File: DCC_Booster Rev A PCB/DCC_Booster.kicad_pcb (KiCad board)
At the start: 2 copper layers, 99.1 x 109.2 mm, 99 parts, among them J1 Conn_01x04, J2 4P4C, J3 4P4C, J4 Prog, J5 Jack-DC, Q1 Q_NMOS_GDS, Q2 Q_NMOS_GDS, Q3 Q_NMOS_GDS, Q4 Q_NMOS_GDS, SW1 SW_DIP_x05, U1 MC34167, U10 LM358, U11 74AHC1G04, U2 R-78E5.0-1.0, U3 74HC08, U4 IR2101, U5 IR2101, U6 74AHC1G04, U7 6N137, U8 PIC16F1847-IP, U9 74AHC1G86

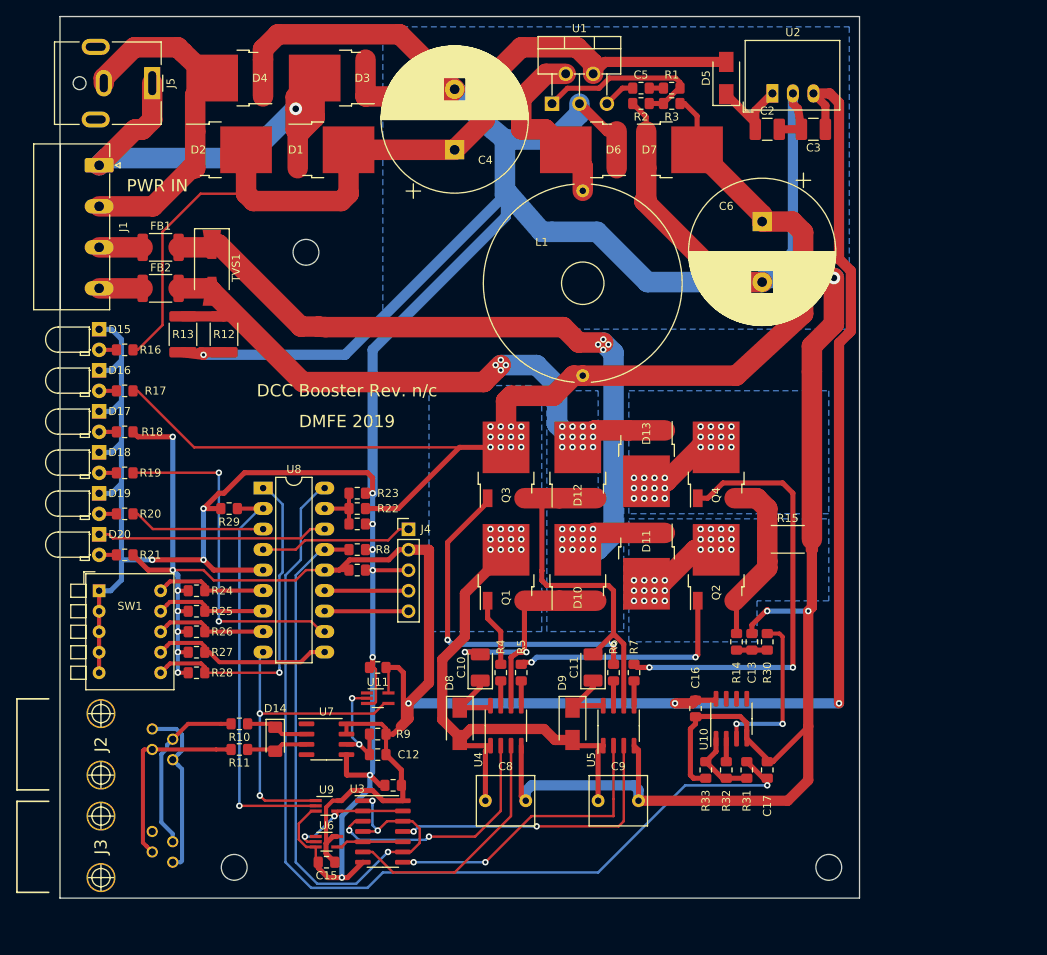
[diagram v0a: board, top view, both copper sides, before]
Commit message: Rev A PCB ordered
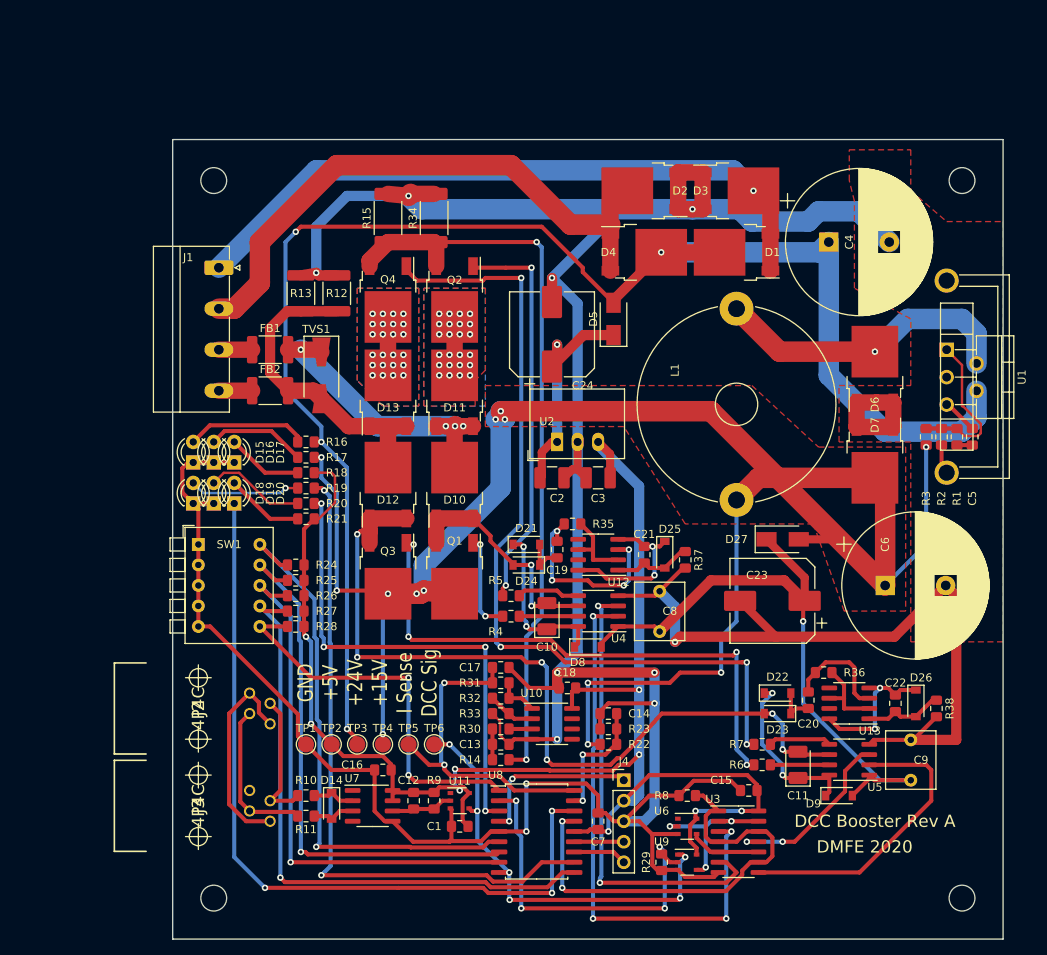
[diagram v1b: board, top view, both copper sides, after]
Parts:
- removed J5: Jack-DC, Connector_BarrelJack:BarrelJack_CUI_PJ-063AH_Horizontal
- added C19: 0.1uf50v, Capacitor_SMD:C_0805_2012Metric_Pad1.15x1.40mm_HandSolder, F.Cu at (97.2, 94.0)
- added C20: 0.1uf50v, Capacitor_SMD:C_0805_2012Metric_Pad1.15x1.40mm_HandSolder, F.Cu at (128.3, 112.6)
- added C21: 0.1uf50v, Capacitor_SMD:C_0805_2012Metric_Pad1.15x1.40mm_HandSolder, F.Cu at (108.0, 94.6)
- added C22: 0.1uf50v, Capacitor_SMD:C_0805_2012Metric_Pad1.15x1.40mm_HandSolder, F.Cu at (139.1, 113.0)
- added C23: 220uF, Capacitor_SMD:CP_Elec_10x10, F.Cu at (123.8, 100.3)
- added C24: 220uF, Capacitor_SMD:CP_Elec_10x10, F.Cu at (96.5, 67.3)
- added D21: 1N4148W, Diode_SMD:D_SOD-123, F.Cu at (93.3, 93.3)
- added D22: 1N4148W, Diode_SMD:D_SOD-123, F.Cu at (124.5, 111.8)
- added D23: 1N4148W, Diode_SMD:D_SOD-123, F.Cu at (124.5, 114.3)
- added D24: 1N4148W, Diode_SMD:D_SOD-123, F.Cu at (93.3, 95.9)
- added D25: BZT52C15, Diode_SMD:D_SOD-123, F.Cu at (110.5, 94.6)
- added D26: BZT52C15, Diode_SMD:D_SOD-123, F.Cu at (141.6, 113.0)
- added D27: MRA4003T3G, Diode_SMD:D_SMA, F.Cu at (125.1, 92.7)
- added H4: MountingHole_3.2mm_M3, MountingHole:MountingHole_3.2mm_M3, F.Cu at (147.3, 137.2)
- added HS1: Heatsink_Fischer_FK224xx2201_25x8.3mm, Heatsink:Heatsink_Fischer_FK224xx2201_25x8.3mm, F.Cu at (145.4, 84.5)
- added R34: 0R10 3W, Resistor_SMD:R_2512_6332Metric_Pad1.52x3.35mm_HandSolder, F.Cu at (81.9, 52.9)
- added R35: 10K, Resistor_SMD:R_0805_2012Metric_Pad1.15x1.40mm_HandSolder, F.Cu at (99.1, 90.8)
- added R36: 10K, Resistor_SMD:R_0805_2012Metric_Pad1.15x1.40mm_HandSolder, F.Cu at (130.2, 109.2)
- added R37: 100, Resistor_SMD:R_0805_2012Metric_Pad1.15x1.40mm_HandSolder, F.Cu at (113.0, 95.2)
- added R38: 100, Resistor_SMD:R_0805_2012Metric_Pad1.15x1.40mm_HandSolder, F.Cu at (144.1, 113.7)
- added TP1: GND, TestPoint:TestPoint_Pad_D2.0mm, F.Cu at (66.0, 118.1)
- added TP2: +5V, TestPoint:TestPoint_Pad_D2.0mm, F.Cu at (69.2, 118.1)
- added TP3: +24V, TestPoint:TestPoint_Pad_D2.0mm, F.Cu at (72.4, 118.1)
- added TP4: +15V, TestPoint:TestPoint_Pad_D2.0mm, F.Cu at (75.6, 118.1)
- added TP5: ISense, TestPoint:TestPoint_Pad_D2.0mm, F.Cu at (78.7, 118.1)
- added TP6: DCC Sig, TestPoint:TestPoint_Pad_D2.0mm, F.Cu at (81.9, 118.1)
- added U12: LM555CM, Package_SO:SOIC-8_3.9x4.9mm_P1.27mm, F.Cu at (102.2, 94.6)
- added U13: LM555CM, Package_SO:SOIC-8_3.9x4.9mm_P1.27mm, F.Cu at (133.3, 113.0)
- D14: footprint Diode_SMD:D_1206_3216Metric_Pad1.42x1.75mm_HandSolder -> Diode_SMD:D_SOD-123
- D15, D16, D17, D18, D19, D20: footprint LED_THT:LED_D3.0mm_Horizontal_O1.27mm_Z2.0mm_Clear -> LED_THT:LED_D3.0mm
- D8, D9: footprint Diode_SMD:D_SMA -> Diode_SMD:D_SOD-123
- L1: footprint Inductor_THT:L_Radial_D24.4mm_P22.90mm_muRATA_1400series -> Inductor_THT:L_Radial_D24.4mm_P23.70mm_muRATA_1400series
- R15: value 0R05 3W -> 0R10 3W
- R32: value 10K -> 100K
- R33: value 20K -> 10K
- U11, U6, U9: footprint Package_TO_SOT_SMD:SOT-353_SC-70-5_Handsoldering -> Package_SO:TSOP-5_1.65x3.05mm_P0.95mm
- U8: footprint Package_DIP:DIP-18_W7.62mm_LongPads -> Package_SO:SOIC-18W_7.5x11.6mm_P1.27mm
- moved H1 114.2 mm to (54.6, 48.3)
- moved H3 81.8 mm to (147.3, 48.3)
- moved R29 69.2 mm to (110.1, 132.7), turned to -90 degrees
- moved R15 63.5 mm to (76.2, 52.9), turned to 90 degrees
- moved C5 59.6 mm to (148.6, 80.0), turned to -90 degrees
- moved U1 57.6 mm to (145.4, 69.2), turned to -90 degrees
- moved R1 55.8 mm to (146.7, 80.0), turned to 90 degrees
- moved R2 55.6 mm to (144.8, 80.0), turned to -90 degrees
- moved U8 54.4 mm to (94.6, 128.9)
- moved D4 53.3 mm to (108.0, 49.5)
- moved C15 53.1 mm to (120.9, 123.8)
- moved D2 53.0 mm to (108.0, 57.1)
- moved D3 52.1 mm to (119.4, 49.5), turned to 0 degrees
- moved R3 51.9 mm to (142.9, 80.0), turned to 90 degrees
- moved D1 51.7 mm to (119.4, 57.1), turned to 180 degrees
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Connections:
- net Net-(C10-Pad1) renamed C10P
- net Net-(C10-Pad2) renamed C10N
- net Net-(C11-Pad1) renamed C11P
- net Net-(C11-Pad2) renamed C11N
- C8 pad 1: +15V -> Vdrive
- C9 pad 1: +15V -> Vdrive
- D8 pad 2: +15V -> Vdrive
- D9 pad 2: +15V -> Vdrive
- Q2 pad 3: Net-(Q2-Pad3) -> GNDS
- Q4 pad 3: Net-(Q2-Pad3) -> GNDS
- R14 pad 1: Net-(Q2-Pad3) -> Net-(C13-Pad1)
- R14 pad 2: Net-(C13-Pad1) -> GNDS
- R15 pad 1: Net-(Q2-Pad3) -> GNDS
- R30 pad 1: Net-(C13-Pad1) -> Net-(R30-Pad1)
- R30 pad 2: Net-(R30-Pad2) -> Net-(C13-Pad1)
- R32 pad 1: Net-(R31-Pad1) -> Net-(R32-Pad1)
- R32 pad 2: Net-(R32-Pad2) -> Net-(R31-Pad1)
- R33 pad 1: GND -> Net-(R32-Pad1)
- R33 pad 2: Net-(R31-Pad1) -> GND
- U10 pad 2: Net-(R32-Pad2) -> Net-(R32-Pad1)
- U10 pad 3: Net-(R30-Pad2) -> Net-(R30-Pad1)
- U4 pad 1: +15V -> Vdrive
- U5 pad 1: +15V -> Vdrive
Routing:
- net GND: track 648.6 -> 523.9 mm, vias 14 -> 11
- net +5V: track 300.8 -> 202.8 mm, vias 10 -> 9
- net GNDS: track 0.00 -> 92.8 mm, vias 0 -> 2
- net +24V: track 110.5 -> 191.4 mm, vias 0 -> 4
- net Vdrive: track 0.00 -> 78.9 mm, vias 0 -> 1
- net Net-(C17-Pad1): track 119.1 -> 41.6 mm, vias 1 -> 2
- net SYSLED: track 28.6 -> 97.9 mm, vias 0 -> 3
- net Net-(D10-Pad2): track 98.9 -> 37.0 mm, vias 16 -> 4
- net C11N: track 46.9 -> 101.9 mm, vias 0 -> 6
- net CurSel0: track 14.1 -> 68.1 mm, vias 0 -> 1
- net Norm/Reverse*: track 22.7 -> 76.0 mm, vias 0 -> 1
- net CurSel1: track 14.1 -> 66.7 mm, vias 0 -> 1
- net CurSel2: track 14.1 -> 65.6 mm, vias 0 -> 1
- net Net-(Q4-Pad1): track 54.5 -> 105.0 mm, vias 2 -> 4
- net DCC_Sig_OK: track 16.9 -> 60.8 mm, vias 0 -> 4
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- added copper zone on F.Cu, net +15V
- added copper zone on F.Cu, net GND
- added copper zone on F.Cu, net Net-(D11-Pad2)
- added copper zone on F.Cu, net Net-(D13-Pad2)
- removed copper zone on B.Cu, net +15V
- removed copper zone on B.Cu, net GND
- removed copper zone on B.Cu, net Net-(D10-Pad2)
- removed copper zone on B.Cu, net Net-(D12-Pad2)
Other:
- board size 99.1 x 109.2 mm -> 102.9 x 99.1 mm
- board text added: "+24V +15V +5V"
- board text added: "DCC Booster Rev A"
- board text added: "DCC OUT"
- board text added: "DMFE 2020"
- board text added: "DRV Sig Sys"
- board text added: "GND +5V +24V +15V I Sense DCC Sig"
- board text removed: "+15V"
- board text removed: "+24V"
- board text removed: "+5V"
- board text removed: "DCC Booster Rev. n/c"
- board text removed: "DCC Sig OK"
- board text removed: "DMFE 2019"
- board text removed: "DRV"
- board text removed: "SYS LED"
